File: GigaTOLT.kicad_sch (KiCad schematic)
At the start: 12 parts

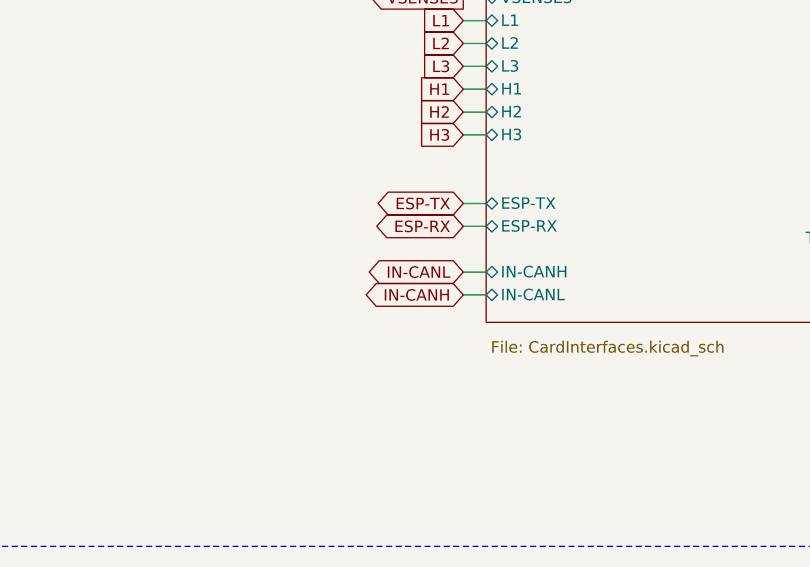
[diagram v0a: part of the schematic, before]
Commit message: initial
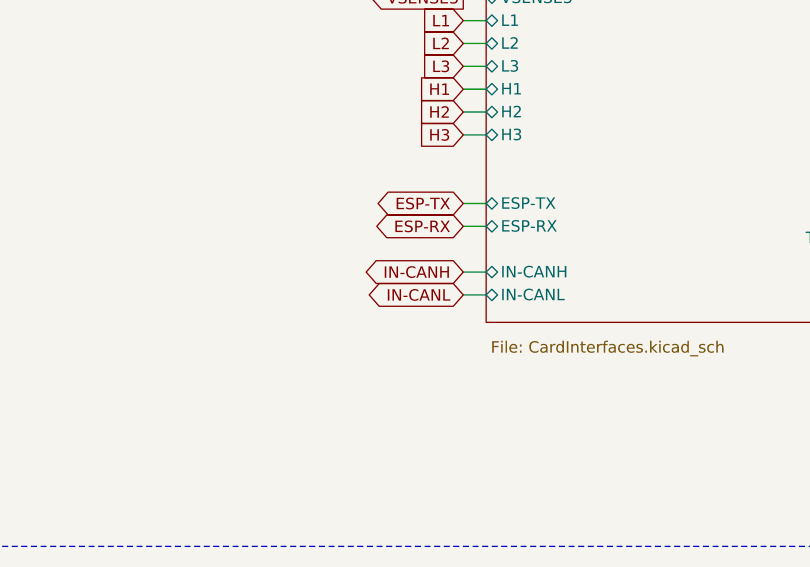
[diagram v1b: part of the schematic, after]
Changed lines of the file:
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@@
 	(global_label "IN-CANL"
 		(shape bidirectional)
-		(at 90.17 236.22 180)
-		(fields_autoplaced yes)
-		(effects
-			(font
-				(size 1.27 1.27)
-			)
-			(justify right)
-		)
-		(property "Intersheetrefs" "${INTERSHEET_REFS}"
-			(at 90.17 236.22 0)
+		(at 90.17 238.76 180)
+		(fields_autoplaced yes)
+		(effects
+			(font
+				(size 1.27 1.27)
+			)
+			(justify right)
+		)
+		(property "Intersheetrefs" "${INTERSHEET_REFS}"
+			(at 90.17 238.76 0)
 			(hide yes)
 			(show_name no)
@@
 	(global_label "IN-CANH"
 		(shape bidirectional)
-		(at 90.17 238.76 180)
-		(fields_autoplaced yes)
-		(effects
-			(font
-				(size 1.27 1.27)
-			)
-			(justify right)
-		)
-		(property "Intersheetrefs" "${INTERSHEET_REFS}"
-			(at 90.17 238.76 0)
-			(hide yes)
-			(show_name no)
+		(at 90.17 236.22 180)
+		(fields_autoplaced yes)
+		(effects
+			(font
+				(size 1.27 1.27)
+			)
+			(justify right)
+		)
+		(property "Intersheetrefs" "${INTERSHEET_REFS}"
+			(at 90.17 236.22 0)
+			(hide yes)
+			(show_name no)

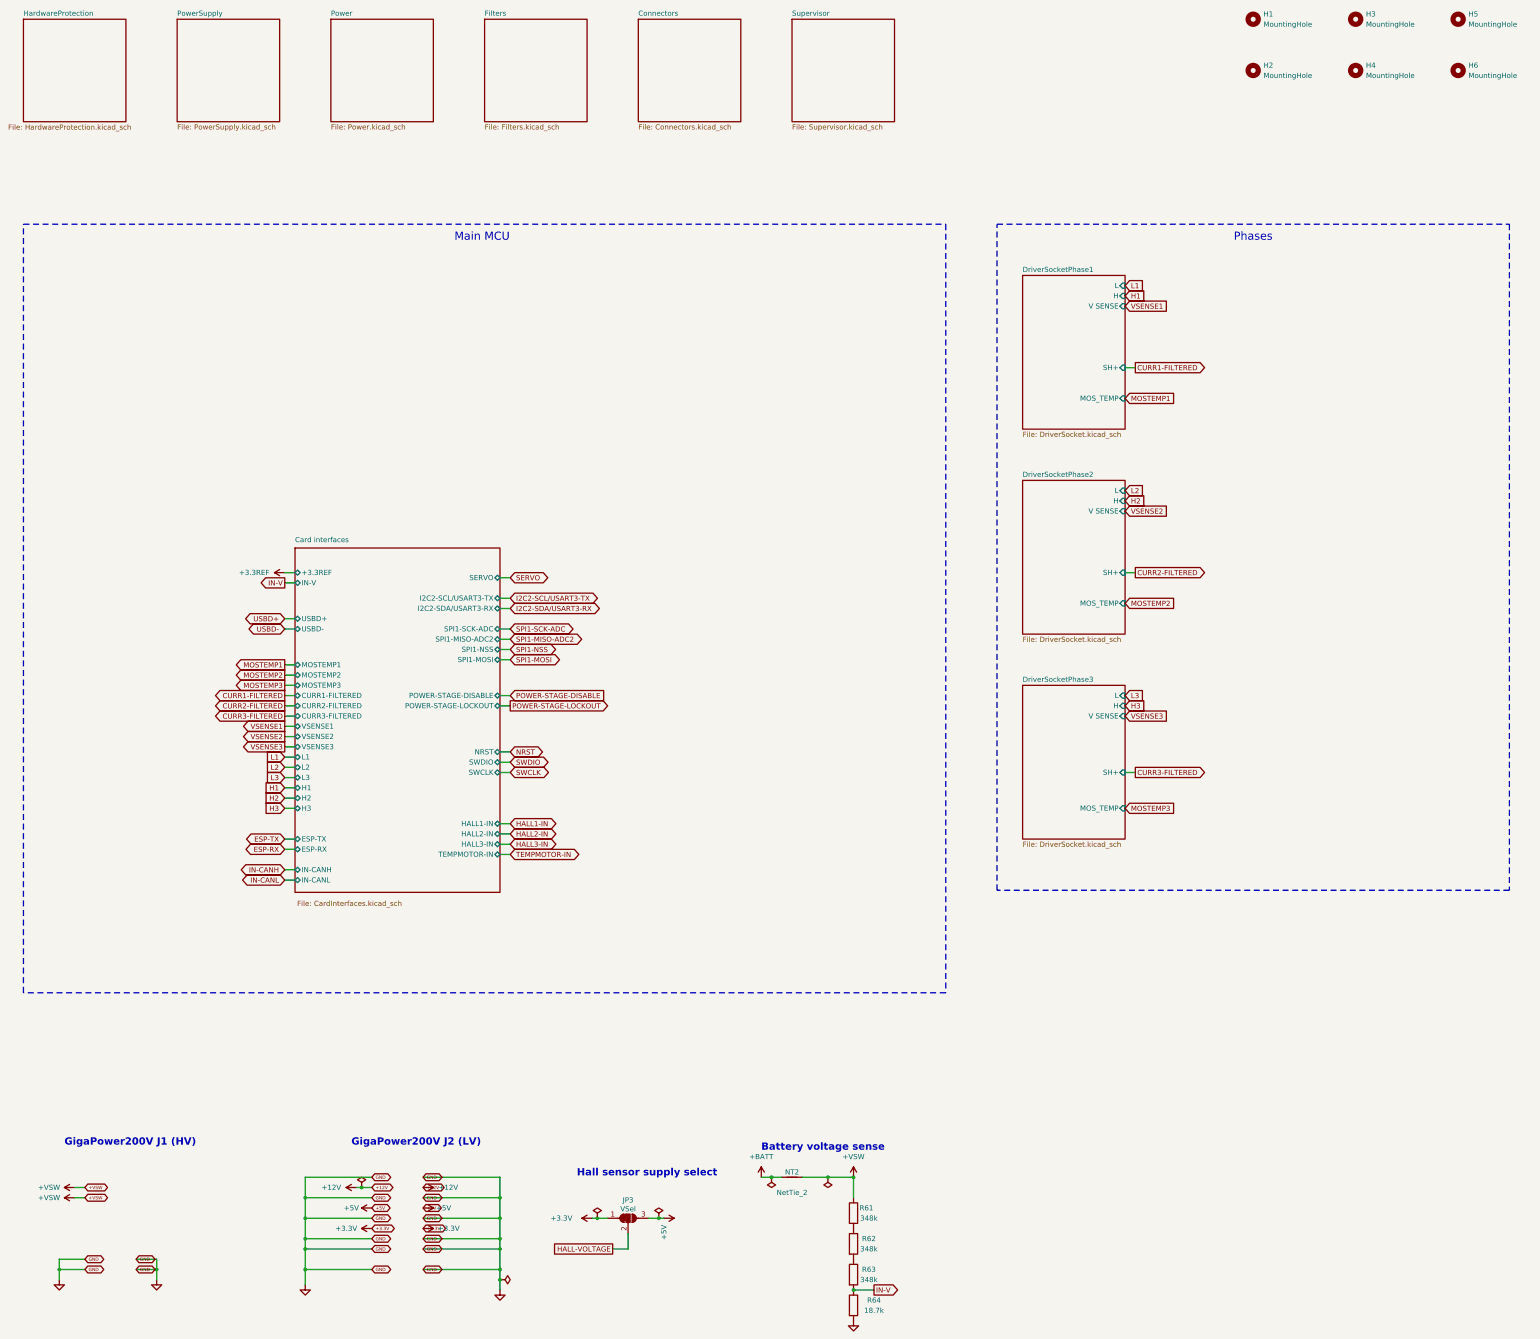
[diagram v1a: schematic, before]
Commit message: initial
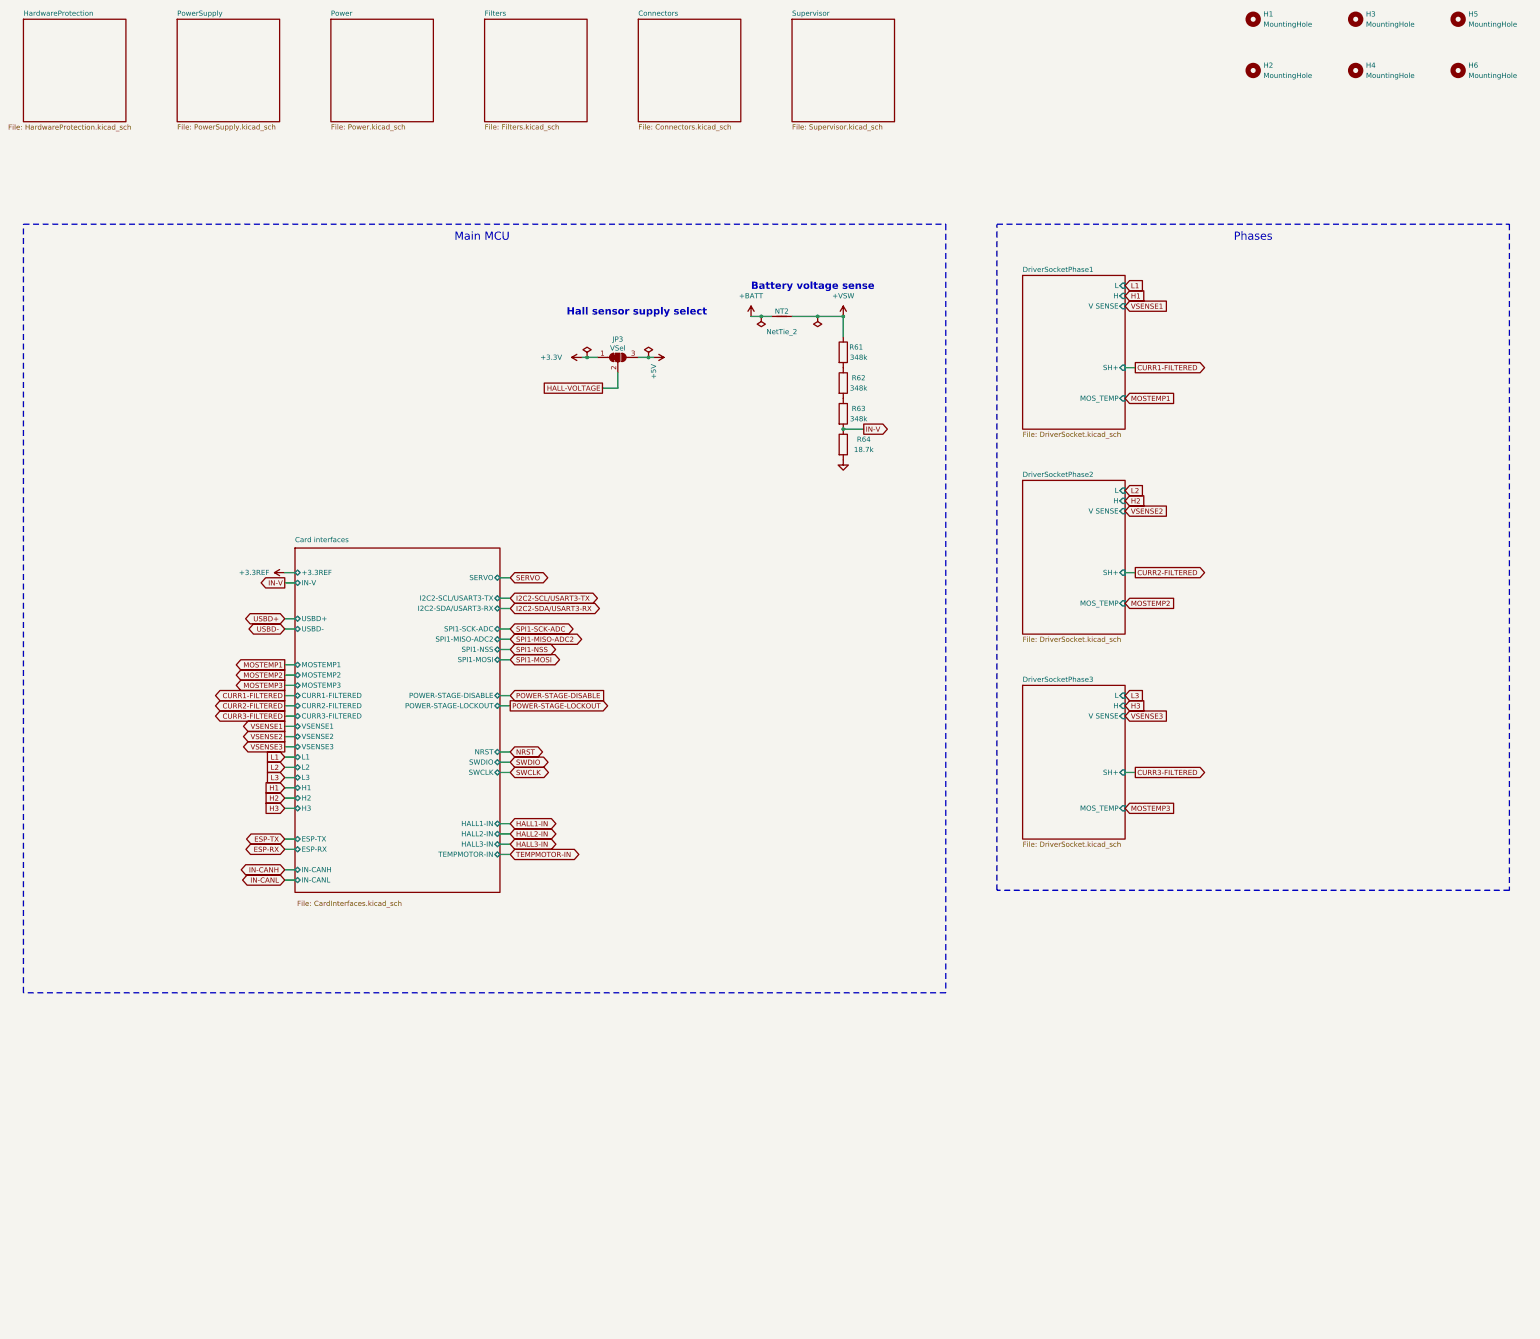
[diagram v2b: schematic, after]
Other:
- note removed: "GigaPower200V J1 (HV)"
- note removed: "GigaPower200V J2 (LV)"
- moved on the sheet: JP3, NT2, R61, R62, R63, R64

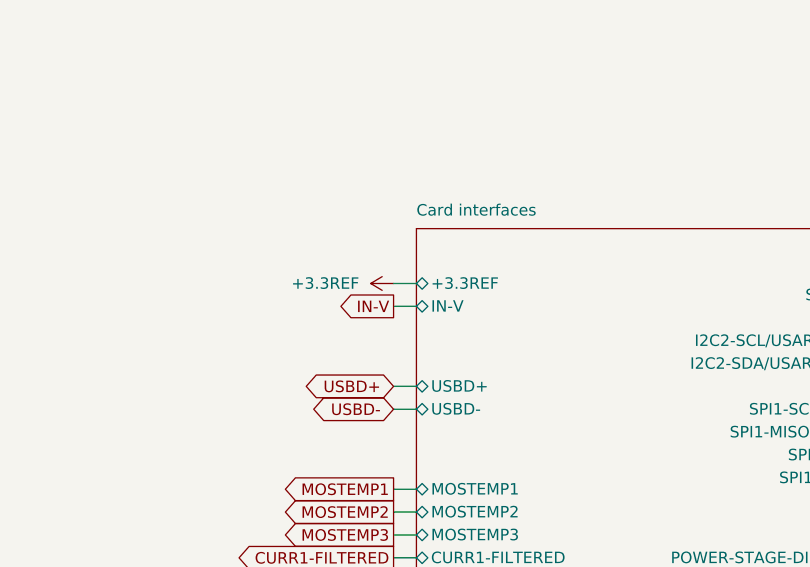
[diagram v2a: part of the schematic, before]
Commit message: clearance
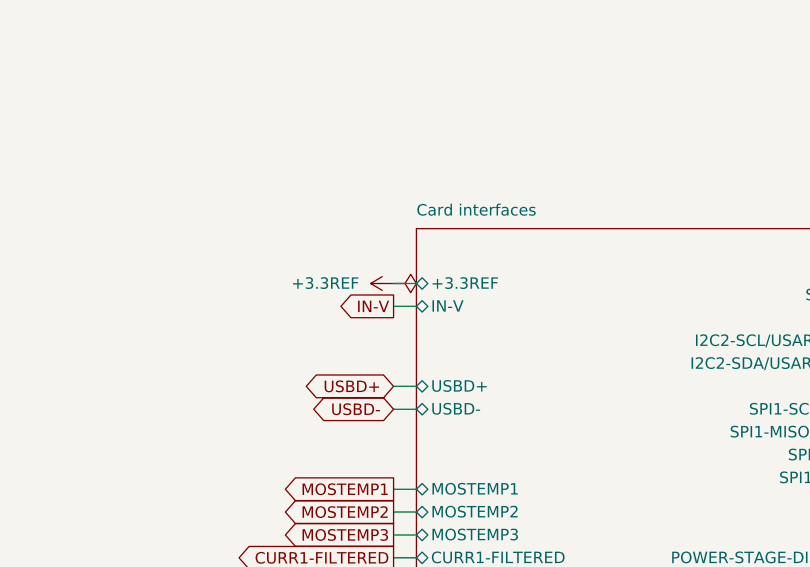
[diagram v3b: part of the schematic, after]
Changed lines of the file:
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@@
+	)
+	(symbol
+		(lib_id "power:PWR_FLAG")
+		(at 90.17 162.56 270)
+		(unit 1)
+		(body_style 1)
+		(exclude_from_sim no)
+		(in_bom yes)
+		(on_board yes)
+		(in_pos_files yes)
+		(dnp no)
+		(fields_autoplaced no)
+		(property "Reference" "#FLG916"
+			(at 90.17 162.56 0)
+			(hide yes)
+			(show_name no)
+			(do_not_autoplace no)
+			(effects
+				(font
+					(size 1.27 1.27)
+				)
+			)
+		)
+		(property "Value" "PWR_FLAG"
+			(at 90.17 162.56 0)
+			(hide yes)
+			(show_name no)
+			(do_not_autoplace no)
+			(effects
+				(font
+					(size 1.27 1.27)
+				)
+			)
+		)
+		(property "Footprint" ""
+			(at 90.17 162.56 0)
+			(hide yes)
+			(show_name no)
+			(do_not_autoplace no)
+			(effects
+				(font
+					(size 1.27 1.27)
+				)
+			)
+		)
+		(property "Datasheet" ""
+			(at 90.17 162.56 0)
+			(hide yes)
+			(show_name no)
+			(do_not_autoplace no)
+			(effects
+				(font
+					(size 1.27 1.27)
+				)
+			)
+		)
+		(property "Description" "Special symbol for telling ERC where power comes from"
+			(at 90.17 162.56 0)
+			(hide yes)
+			(show_name no)
+			(do_not_autoplace no)
+			(effects
+				(font
+					(size 1.27 1.27)
+				)
+			)
+		)
+		(pin "1"
+		)
+		(instances
+			(project "GigaTOLT"
+				(path "/768a484b-8a27-40cf-8cad-0f63935b1af0"
+					(reference "#FLG916")
+					(unit 1)
+				)
+			)
+		)
 	)
 	(symbol
